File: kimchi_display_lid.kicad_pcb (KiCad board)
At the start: 4 copper layers, 65 x 32 mm, 8 parts, among them J1 DF40HC(3.5)-60DS, J2 DF40HC(3.5)-60DS, U1 24C32

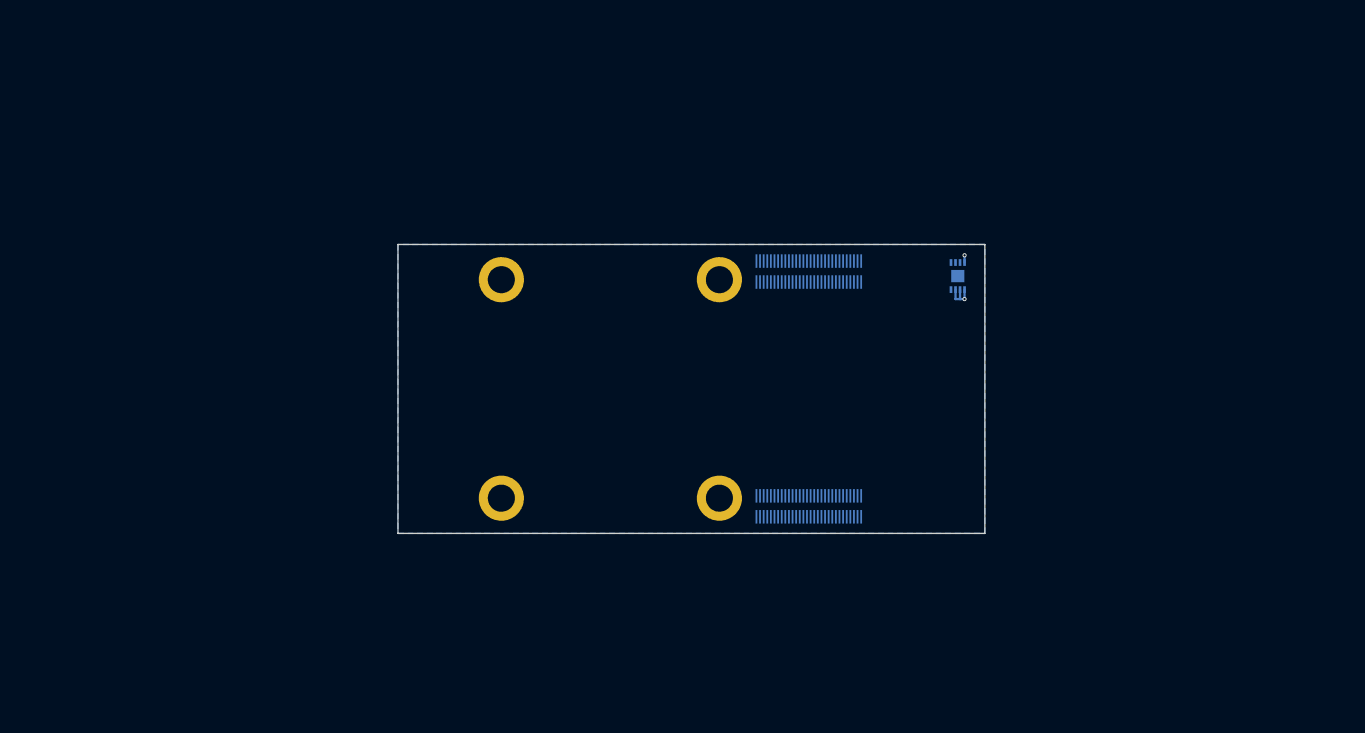
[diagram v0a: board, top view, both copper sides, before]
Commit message: Add board outline
Signed-off-by: Michael Welling <mwelling@ieee.org>
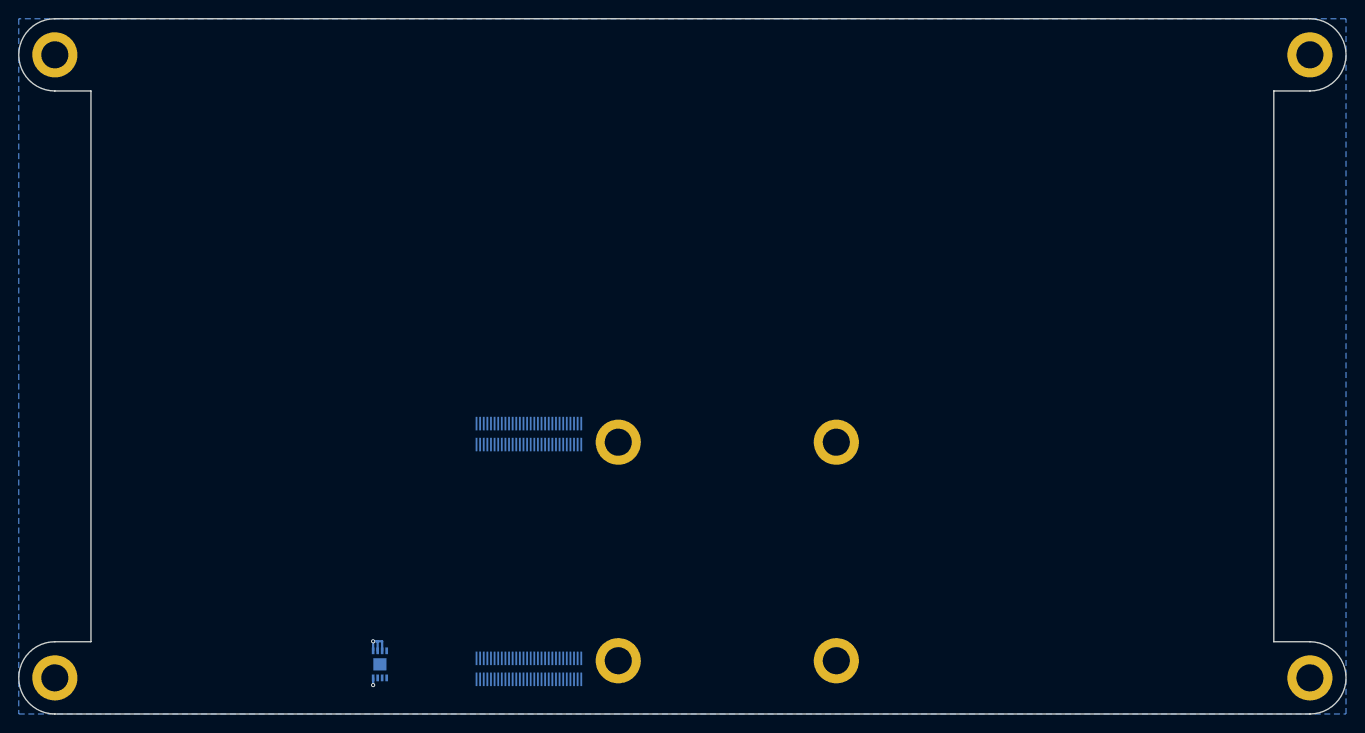
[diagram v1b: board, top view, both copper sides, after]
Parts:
- added H5: MountingHole_Pad, kimchi_ulid:MountingHole_3mm_Pad, F.Cu at (69.0, 142.0)
- added H6: MountingHole_Pad, kimchi_ulid:MountingHole_3mm_Pad, F.Cu at (69.0, 73.0)
- added H7: MountingHole_Pad, kimchi_ulid:MountingHole_3mm_Pad, F.Cu at (208.0, 73.0)
- added H8: MountingHole_Pad, kimchi_ulid:MountingHole_3mm_Pad, F.Cu at (208.0, 142.0)
- moved LOGO1 88.4 mm to (198.0, 140.0)
- moved U1 77.1 mm to (105.0, 140.5), turned to 270 degrees
- moved H1 56.2 mm to (155.6, 140.1), turned to 180 degrees
- moved J1 53.8 mm to (121.5, 141.0), turned to 0 degrees
- moved H3 43.7 mm to (131.4, 140.1), turned to 180 degrees
- moved H2 37.6 mm to (155.6, 115.9), turned to 180 degrees
- moved J2 32.0 mm to (121.5, 115.0), turned to 0 degrees
- moved H4 12.8 mm to (131.4, 115.9), turned to 180 degrees
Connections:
- J1 pad 1: (no net) -> /USDHC3_CMD
- J1 pad 17: (no net) -> I2C3_SDA
- J1 pad 18: (no net) -> I2C3_SCL
- J1 pad 19: (no net) -> I2C2_SDA
- J1 pad 2: (no net) -> /USDHC3_CLK
- J1 pad 20: (no net) -> I2C2_SCL
- J1 pad 21: (no net) -> I2C1_SDA
- J1 pad 22: (no net) -> I2C1_SCL
- J1 pad 23: (no net) -> ECSPI1_SCLK
- J1 pad 24: (no net) -> ECSPI1_SS0
- J1 pad 25: (no net) -> ECSPI1_MOSI
- J1 pad 26: (no net) -> ECSPI1_MISO
- J1 pad 27: (no net) -> ECSPI2_SCLK
- J1 pad 28: (no net) -> ECSPI2_SS0
- J1 pad 29: (no net) -> ECSPI2_MOSI
- J1 pad 3: (no net) -> /USDHC3_DATA3
- J1 pad 30: (no net) -> ECSPI2_MISO
- J1 pad 31: (no net) -> /DISP_D0_N
- J1 pad 32: (no net) -> /DISP_D0_P
- J1 pad 33: (no net) -> /DISP_D1_N
- J1 pad 34: (no net) -> /DISP_D1_P
- J1 pad 35: (no net) -> /DISP_CK_N
- J1 pad 36: (no net) -> /DISP_CK_P
- J1 pad 37: (no net) -> /DISP_D2_N
- J1 pad 38: (no net) -> /DISP_D2_P
- J1 pad 39: (no net) -> /DISP_D3_N
- J1 pad 4: (no net) -> /USDHC3_DATA0
- J1 pad 40: (no net) -> /DISP_D3_P
- J1 pad 41: (no net) -> /CAM_D0_N
- J1 pad 42: (no net) -> /CAM_D0_P
- J1 pad 43: (no net) -> /CAM_D1_N
- J1 pad 44: (no net) -> /CAM_D1_P
- J1 pad 45: (no net) -> /CAM_CK_N
- J1 pad 46: (no net) -> /CAM_CK_P
- J1 pad 47: (no net) -> /CAM_D2_N
- J1 pad 48: (no net) -> /CAM_D2_P
- J1 pad 49: (no net) -> /CAM_D3_N
- J1 pad 5: (no net) -> /USDHC3_DATA1
- J1 pad 50: (no net) -> /CAM_D3_P
- J1 pad 52: (no net) -> UIM_VPP
- J1 pad 53: (no net) -> UIM_RESET_N
- J1 pad 54: (no net) -> UIM_CLK
- J1 pad 55: (no net) -> UIM_DATA
- J1 pad 56: (no net) -> UIM_PWR
- J1 pad 57: (no net) -> USB2_VBUS
- J1 pad 58: (no net) -> USB2_ID
- J1 pad 59: (no net) -> USB2_DN
- J1 pad 6: (no net) -> /USDHC3_DATA2
- J1 pad 60: (no net) -> USB2_DP
- J2 pad 1: (no net) -> /ENET_MDIO
- J2 pad 10: (no net) -> /ENET_TD0
- J2 pad 11: (no net) -> /ENET_TD3
- J2 pad 12: (no net) -> /ENET_TD2
- J2 pad 13: (no net) -> /ENET_TX_CTL
- J2 pad 14: (no net) -> /ENET_TXC
- J2 pad 15: (no net) -> SAI2_RXD0
- J2 pad 16: (no net) -> SAI2_TXFS
- J2 pad 17: (no net) -> SAI2_RXC
- J2 pad 18: (no net) -> SAI2_TXD0
- J2 pad 19: (no net) -> SAI2_TXC
- J2 pad 2: (no net) -> /ENET_MDC
- J2 pad 20: (no net) -> SAI2_MCLK
- J2 pad 21: (no net) -> SAI2_RXFS
- J2 pad 22: (no net) -> GPIO1[15]
- J2 pad 23: (no net) -> GPIO1[14]
- J2 pad 24: (no net) -> GPIO1[13]
- J2 pad 25: (no net) -> GPIO1[12]
- J2 pad 26: (no net) -> GPIO1[11]
- J2 pad 27: (no net) -> GPIO1[10]
- J2 pad 28: (no net) -> GPIO1[9]
- J2 pad 29: (no net) -> GPIO1[1]
- J2 pad 3: (no net) -> /ENET_RD3
- J2 pad 30: (no net) -> GPIO1[0]
- J2 pad 31: (no net) -> SAI3_TXC
- J2 pad 32: (no net) -> SAI3_TXD
- J2 pad 33: (no net) -> SAI3_RXD
- J2 pad 34: (no net) -> SAI3_RXFS
- J2 pad 35: (no net) -> SAI3_RXC
- J2 pad 36: (no net) -> SAI3_TXFS
- J2 pad 37: (no net) -> SAI3_MCLK
- J2 pad 4: (no net) -> /ENET_RD1
- J2 pad 46: (no net) -> UART1_TX
- J2 pad 47: (no net) -> UART1_RX
- J2 pad 48: (no net) -> UART3_TX
- J2 pad 49: (no net) -> UART3_RX
- J2 pad 5: (no net) -> /ENET_RD2
- J2 pad 58: (no net) -> Net-(J2-Pad58)
- J2 pad 59: (no net) -> PCIE_USB_D_P
- J2 pad 6: (no net) -> /ENET_RD0
- J2 pad 60: (no net) -> PCIE_USB_D_N
- J2 pad 7: (no net) -> /ENET_RXC
- J2 pad 8: (no net) -> /ENET_RX_CTL
- J2 pad 9: (no net) -> /ENET_TD1
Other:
- board size 65 x 32 mm -> 147 x 77 mm
- board text added: "USB C"

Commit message: Add 3D model for the kimchi micro
The PEMs are supposed to be 3.5mm but the spacing is enforced in the footprint.

Signed-off-by: Michael Welling <mwelling@ieee.org>
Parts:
- added REF**: kimchi-micro-3d-model, kimchi_ulid:kimchi-micro-3d-model, B.Cu at (134.5, 128.0)
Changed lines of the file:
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@@
     (tracks 8)
     (zones 0)
-    (modules 12)
+    (modules 13)
     (nets 100)
   )
@@
       (xy -1.971615 -1.454739) (xy -1.908759 -1.469184)) (layer B.SilkS) (width 0.01))
   )
+  (module kimchi_ulid:kimchi-micro-3d-model (layer B.Cu)
+    (at 134.5 128)
+    (fp_text reference REF** (at 29.75 14.75) (layer B.SilkS)
+      (effects (font (size 1 1) (thickness 0.15)) (justify mirror))
+    )
+    (fp_text value kimchi-micro-3d-model (at 0 0.5) (layer B.Fab)
+      (effects (font (size 1 1) (thickness 0.15)) (justify mirror))
+    )
+    (fp_line (start -32.5 16) (end -32.5 -16) (layer B.SilkS) (width 0.08))
+    (fp_line (start 32.5 16) (end -32.5 16) (layer B.SilkS) (width 0.08))
+    (fp_line (start 32.5 -16) (end 32.5 16) (layer B.SilkS) (width 0.08))
+    (fp_line (start -32.5 -16) (end 32.5 -16) (layer B.SilkS) (width 0.08))
+    (model ${KIPRJMOD}/3D/kimchi_micro.step
+      (offset (xyz 32.5 -16 4.25))
+      (scale (xyz 1 1 1))
+      (rotate (xyz 0 180 0))
+    )
+  )
   (gr_text "USB C" (at 141 143) (layer B.SilkS)
     (effects (font (size 1.5 1.5) (thickness 0.3)) (justify mirror))
@@
     (connect_pads (clearance 0.127))
     (min_thickness 0.127)
-    (fill yes (arc_segments 32) (thermal_gap 0.127) (thermal_bridge_width 1.27))
+    (fill (arc_segments 32) (thermal_gap 0.127) (thermal_bridge_width 1.27))
     (polygon
       (pts
@@
     (connect_pads (clearance 0.127))
     (min_thickness 0.127)
-    (fill yes (arc_segments 32) (thermal_gap 0.127) (thermal_bridge_width 0.508))
+    (fill (arc_segments 32) (thermal_gap 0.127) (thermal_bridge_width 0.508))
     (polygon
       (pts
@@
     (connect_pads (clearance 0.127))
     (min_thickness 0.254)
-    (fill yes (arc_segments 32) (thermal_gap 0.508) (thermal_bridge_width 0.508))
+    (fill (arc_segments 32) (thermal_gap 0.508) (thermal_bridge_width 0.508))
     (polygon
       (pts
